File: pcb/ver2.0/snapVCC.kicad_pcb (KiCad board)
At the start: 2 copper layers, 25.9 x 17.3 mm, 26 parts, among them P1 CONN_01X03, P2 CONN_01X02, Q1 IRLML9301TRPbF, U1 TPS560200

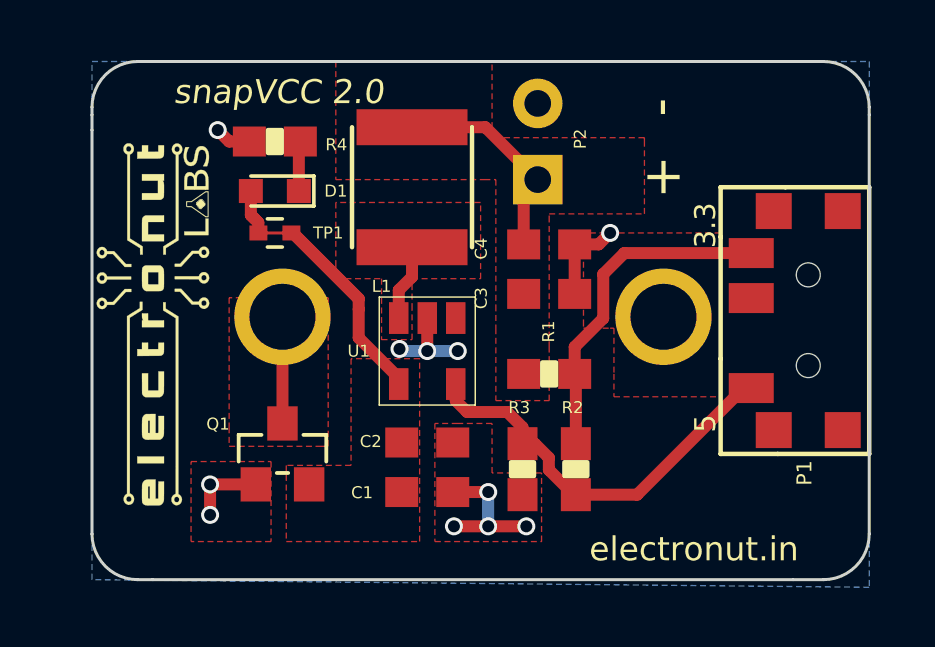
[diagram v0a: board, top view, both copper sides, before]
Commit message: gerbers updated
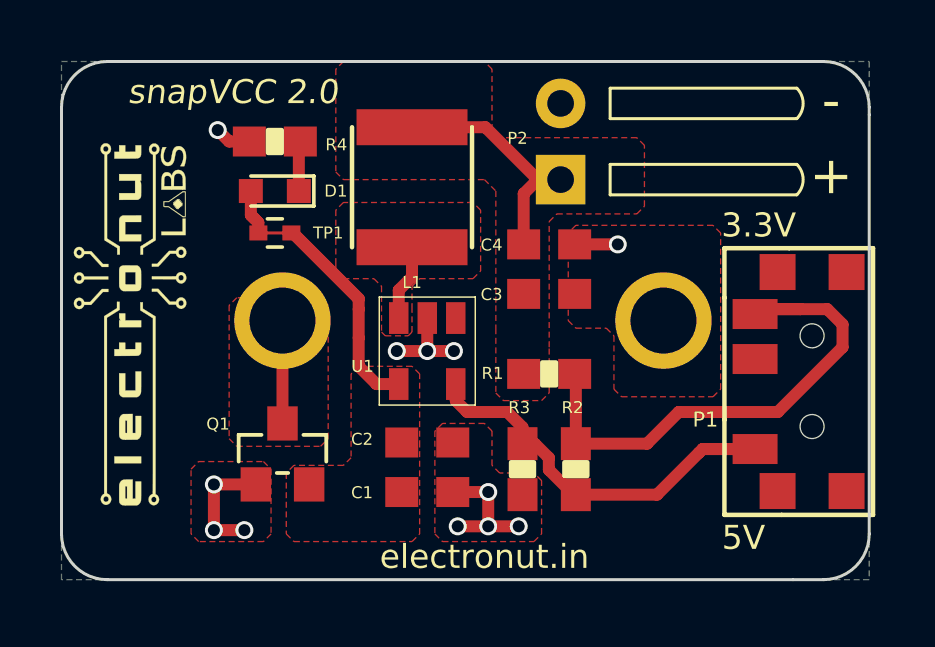
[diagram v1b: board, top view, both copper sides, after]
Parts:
- moved P1 2.04 mm to (159.6, 107.2)
- moved G*** 0.76 mm to (136.9, 105.3)
- moved P2 0.76 mm to (151.3, 99.2)
- moved BT1 0.13 mm to (148.3, 105.2)
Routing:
- net Net-(P1-Pad3): track 11.3 -> 18.7 mm
- net GND: track 15.9 -> 14.2 mm, vias 11 -> 12
- net Net-(P1-Pad1): track 13.7 -> 14.6 mm
- net Net-(C1-Pad1): track 11.4 -> 12.0 mm
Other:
- board size 25.9 x 17.3 mm -> 26.9 x 17.3 mm
- board text added: "3.3V"
- board text added: "5V"
- board text removed: "3.3"
- board text removed: "5"

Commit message: gerbers changes updated
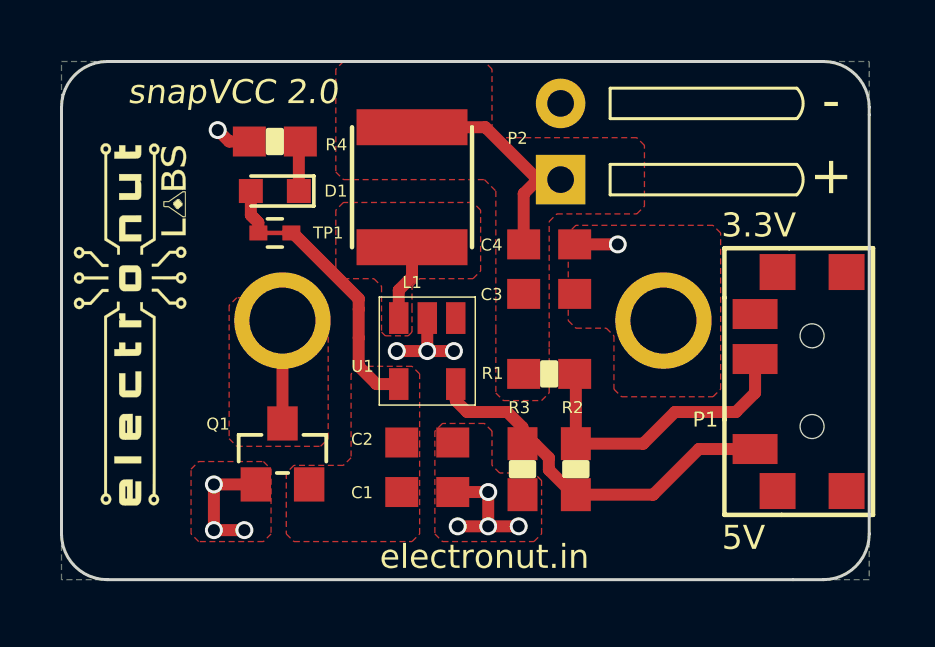
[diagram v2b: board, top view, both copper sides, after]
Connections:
- R1 pad 2: Net-(P1-Pad3) -> Net-(P1-Pad2)
- R2 pad 1: Net-(P1-Pad3) -> Net-(P1-Pad2)
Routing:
- net Net-(P1-Pad3): track 18.7 -> 0.92 mm
- net Net-(P1-Pad2): track 0.00 -> 10.1 mm
- net Net-(P1-Pad1): track 14.6 -> 13.0 mm
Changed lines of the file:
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@@
     (thickness 0.8)
     (drawings 25)
-    (tracks 80)
+    (tracks 74)
     (zones 0)
     (modules 26)
@@
       (net 4 "Net-(C3-Pad1)"))
     (pad 2 smd rect (at 0.85 0) (size 1.1 1) (layers F.Cu F.Paste F.Mask)
-      (net 6 "Net-(P1-Pad3)"))
+      (net 8 "Net-(P1-Pad2)"))
   )
   (module snapVCC_lib:0603-RES (layer F.Cu)
@@
     (fp_poly (pts (xy -0.2286 0.381) (xy 0.2286 0.381) (xy 0.2286 -0.381) (xy -0.2286 -0.381)) (layer F.SilkS) (width 0.15))
     (pad 1 smd rect (at -0.85 0 270) (size 1.1 1) (layers F.Cu F.Paste F.Mask)
-      (net 6 "Net-(P1-Pad3)"))
+      (net 8 "Net-(P1-Pad2)"))
     (pad 2 smd rect (at 0.85 0 270) (size 1.1 1) (layers F.Cu F.Paste F.Mask)
       (net 7 "Net-(P1-Pad1)"))
@@
     (pad 1 smd rect (at 0.55 0) (size 0.6 0.5) (layers F.Cu F.Paste F.Mask)
       (net 3 "Net-(C1-Pad1)"))
-    (pad 1 smd rect (at 0 0) (size 0.8 0.1) (layers F.Cu F.Paste F.Mask)
+    (pad 1 smd rect (at 0 0) (size 0.8 0.15) (layers F.Cu F.Paste F.Mask)
       (net 3 "Net-(C1-Pad1)"))
   )
@@
   (segment (start 145.862 105.072) (end 145.862 104.142) (width 0.4) (layer F.Cu) (net 5))
   (segment (start 145.862 104.142) (end 146.304 103.7) (width 0.4) (layer F.Cu) (net 5))
-  (segment (start 159.258 104.775) (end 157.902 104.775) (width 0.4) (layer F.Cu) (net 6))
   (segment (start 157.902 104.775) (end 157.739 104.938) (width 0.4) (layer F.Cu) (net 6))
-  (segment (start 151.765 109.259) (end 154.139 109.259) (width 0.4) (layer F.Cu) (net 6))
-  (segment (start 160.147 104.775) (end 159.258 104.775) (width 0.4) (layer F.Cu) (net 6))
-  (segment (start 159.258 104.775) (end 157.775 104.775) (width 0.4) (layer F.Cu) (net 6))
-  (segment (start 160.655 105.283) (end 160.147 104.775) (width 0.4) (layer F.Cu) (net 6))
-  (segment (start 160.655 106.045) (end 160.655 105.283) (width 0.4) (layer F.Cu) (net 6))
-  (segment (start 158.496 108.204) (end 160.655 106.045) (width 0.4) (layer F.Cu) (net 6))
-  (segment (start 155.194 108.204) (end 158.496 108.204) (width 0.4) (layer F.Cu) (net 6))
-  (segment (start 154.139 109.259) (end 155.194 108.204) (width 0.4) (layer F.Cu) (net 6))
   (segment (start 157.775 104.775) (end 157.612 104.938) (width 0.4) (layer F.Cu) (net 6))
   (segment (start 157.775 104.902) (end 157.612 105.065) (width 0.4) (layer F.Cu) (net 6))
   (segment (start 157.775 104.902) (end 157.612 105.065) (width 0.4) (layer F.Cu) (net 6))
-  (segment (start 151.765 109.259) (end 151.765 106.973) (width 0.4) (layer F.Cu) (net 6))
-  (segment (start 151.765 106.973) (end 151.726 106.934) (width 0.4) (layer F.Cu) (net 6))
-  (segment (start 157.739 109.438) (end 155.992 109.438) (width 0.4) (layer F.Cu) (net 7))
-  (segment (start 157.612 109.438) (end 155.992 109.438) (width 0.4) (layer F.Cu) (net 7))
-  (segment (start 155.992 109.438) (end 155.865 109.565) (width 0.4) (layer F.Cu) (net 7))
-  (segment (start 151.765 110.959) (end 154.471 110.959) (width 0.4) (layer F.Cu) (net 7))
-  (segment (start 154.471 110.959) (end 155.865 109.565) (width 0.4) (layer F.Cu) (net 7))
+  (segment (start 157.739 109.438) (end 155.865 109.438) (width 0.4) (layer F.Cu) (net 7))
+  (segment (start 154.344 110.959) (end 151.765 110.959) (width 0.4) (layer F.Cu) (net 7))
+  (segment (start 155.865 109.438) (end 154.344 110.959) (width 0.4) (layer F.Cu) (net 7))
   (segment (start 147.762 107.272) (end 147.762 107.823) (width 0.4) (layer F.Cu) (net 7))
   (segment (start 147.762 107.823) (end 148.143 108.204) (width 0.4) (layer F.Cu) (net 7))
@@
   (segment (start 149.987 109.259) (end 150.395999 109.259) (width 0.4) (layer F.Cu) (net 7))
   (segment (start 150.395999 109.259) (end 150.864999 109.728) (width 0.4) (layer F.Cu) (net 7))
+  (segment (start 151.765 109.259) (end 154.012 109.259) (width 0.4) (layer F.Cu) (net 8))
+  (segment (start 157.739 107.564) (end 157.739 106.438) (width 0.4) (layer F.Cu) (net 8))
+  (segment (start 157.099 108.204) (end 157.739 107.564) (width 0.4) (layer F.Cu) (net 8))
+  (segment (start 155.067 108.204) (end 157.099 108.204) (width 0.4) (layer F.Cu) (net 8))
+  (segment (start 154.012 109.259) (end 155.067 108.204) (width 0.4) (layer F.Cu) (net 8))
+  (segment (start 151.765 109.259) (end 151.765 106.973) (width 0.4) (layer F.Cu) (net 8))
+  (segment (start 151.765 106.973) (end 151.726 106.934) (width 0.4) (layer F.Cu) (net 8))
   (segment (start 142.532 100.838) (end 142.532 99.237) (width 0.4) (layer F.Cu) (net 9))
   (segment (start 142.532 99.237) (end 142.582 99.187) (width 0.4) (layer F.Cu) (net 9))
